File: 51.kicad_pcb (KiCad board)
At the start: 2 copper layers, 30.5 x 35.6 mm, 4 parts, among them J1 USB_C_Receptacle_USB2.0, J2 Conn_01x11, J3 Conn_01x11

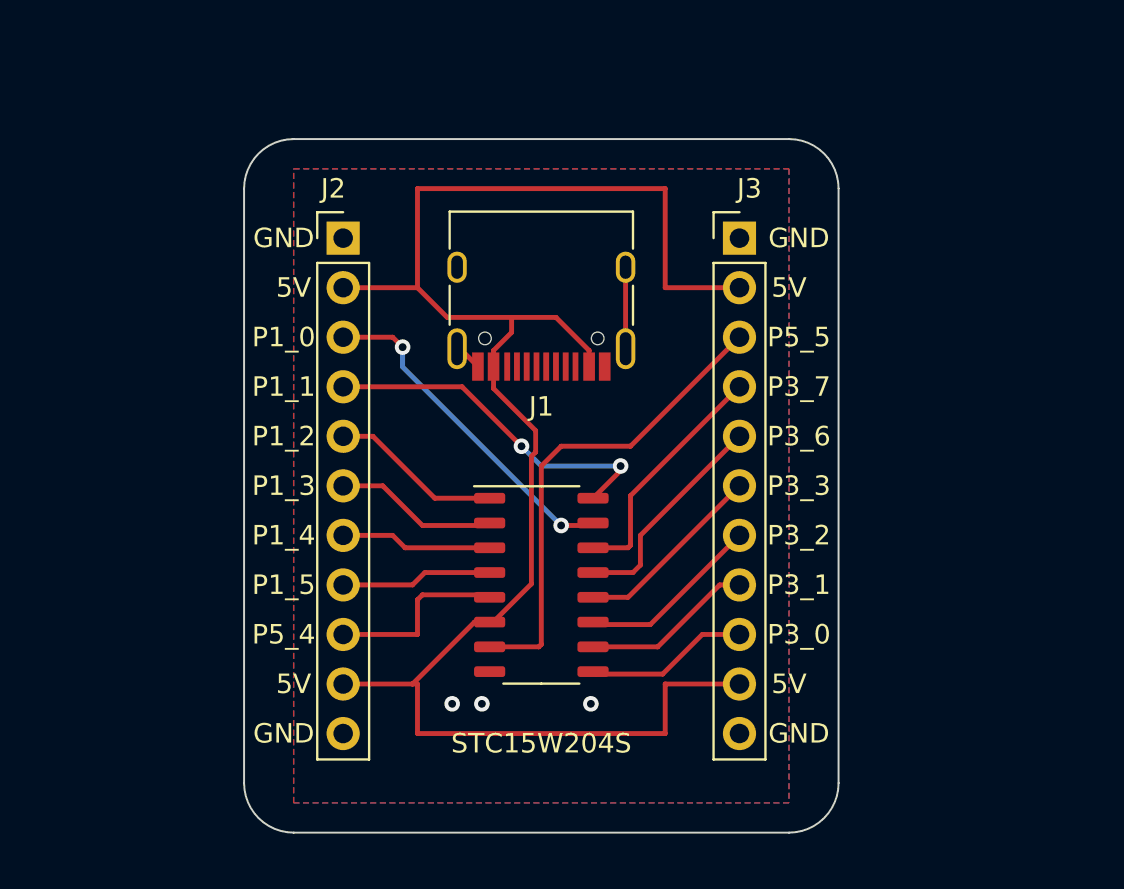
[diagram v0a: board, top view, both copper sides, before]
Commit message: add switch */ /
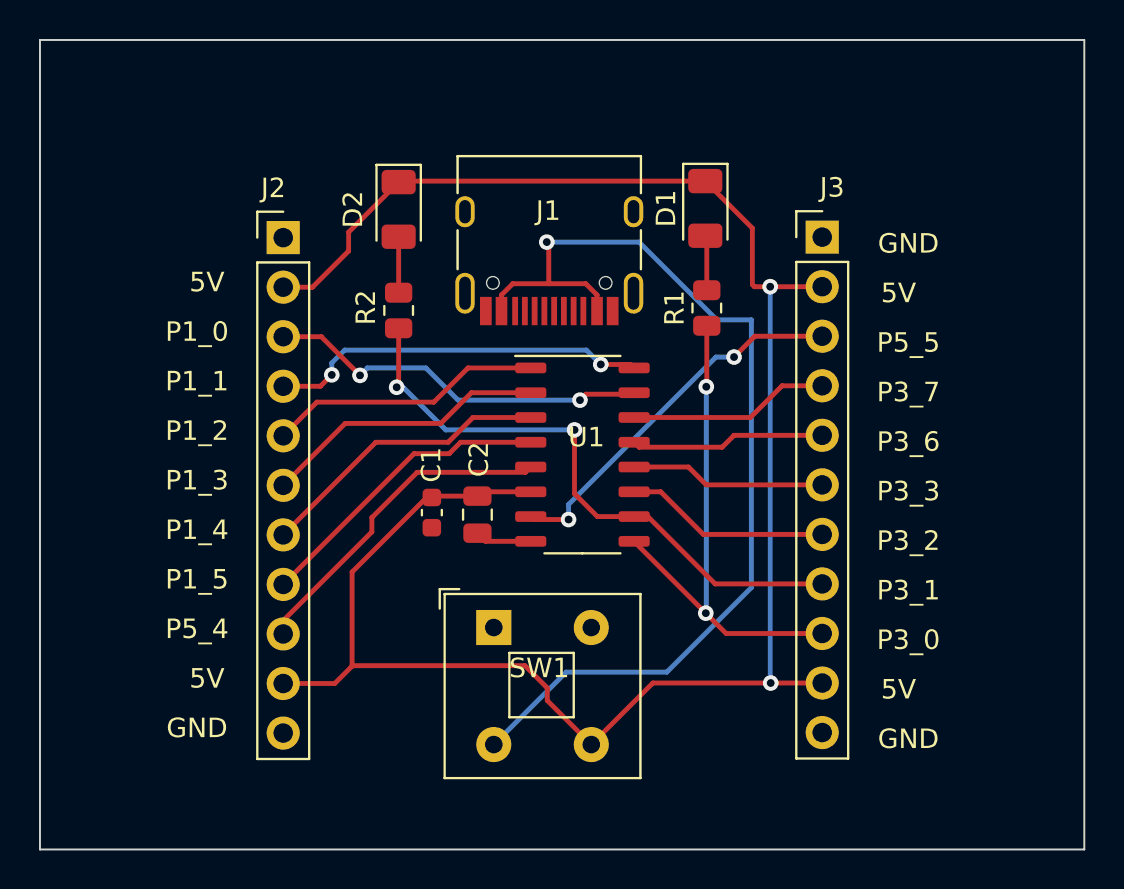
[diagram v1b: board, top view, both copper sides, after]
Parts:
- removed STC15W204S: STC15W204S-35x-SOP16, Package_SO:STC_SOP-16_3.9x9.9mm_P1.27mm
- added C1: 47uF, Capacitor_SMD:C_0603_1608Metric, F.Cu at (106.1, 67.4)
- added C2: 0.1uF, Capacitor_SMD:C_0805_2012Metric, F.Cu at (108.5, 67.5)
- added D1: LED, LED_SMD:LED_1206_3216Metric, F.Cu at (120.2, 51.8)
- added D2: LED, LED_SMD:LED_1206_3216Metric, F.Cu at (104.4, 51.9)
- added R1: R, Resistor_SMD:R_0805_2012Metric, F.Cu at (120.2, 56.9)
- added R2: R, Resistor_SMD:R_0805_2012Metric, F.Cu at (104.4, 57.0)
- added SW1: SW_DPST, Button_Switch_THT:SW_Push_2P1T_Toggle_CK_PVA1xxH4xxxxxxV2, F.Cu at (109.3, 73.3)
- added U1: STC15W204S-35x-SOP16, Package_SO:STC_SOP-16_3.9x9.9mm_P1.27mm, F.Cu at (113.9, 64.4)
- moved J3 4.24 mm to (126.2, 53.3)
- moved J2 3.07 mm to (98.5, 53.3)
- moved J1 2.87 mm to (112.2, 53.0)
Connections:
- J2 pad 1: GND -> GND1
- J2 pad 10: +5V -> VCC
- J2 pad 11: GND -> GND1
- J2 pad 2: +5V -> VCC
- J3 pad 1: GND -> GND1
- J3 pad 10: +5V -> VCC
- J3 pad 11: GND -> GND1
- J3 pad 2: +5V -> VCC
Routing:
- net VCC: track 0.00 -> 101.8 mm, vias 0 -> 2
- net +5V: track 90.1 -> 51.6 mm, vias 0 -> 1
- net p3_1: track 8.83 -> 31.0 mm, vias 0 -> 2
- net p3_0: track 8.40 -> 26.4 mm, vias 0 -> 2
- net p1_5: track 7.77 -> 15.7 mm
- net p5_4: track 9.45 -> 17.1 mm
- net p1_4: track 7.77 -> 15.2 mm
- net p1_3: track 8.40 -> 14.7 mm
- net GND: track 5.63 -> 0.00 mm, vias 3 -> 0
- net p5_5: track 24.7 -> 19.4 mm, vias 0 -> 2
- net p1_2: track 8.83 -> 14.1 mm
- net GND1: track 0.00 -> 2.91 mm
- net Net-(D2-Pad2): track 0.00 -> 2.87 mm
- net Net-(D1-Pad2): track 0.00 -> 2.82 mm
- net p1_0: track 17.5 -> 19.8 mm
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- removed copper zone on B.Cu, net GND
- removed copper zone on F.Cu, net GND
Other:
- board size 30.5 x 35.6 mm -> 53.5 x 41.5 mm
